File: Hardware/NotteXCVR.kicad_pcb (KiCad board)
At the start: 2 copper layers, 20.3 x 8.4 mm, 8 parts, among them J1 Bus_PCI_Express_x1, J2 GMI-10-2-1.27-G-10, U2 XC7A35T-CSG325

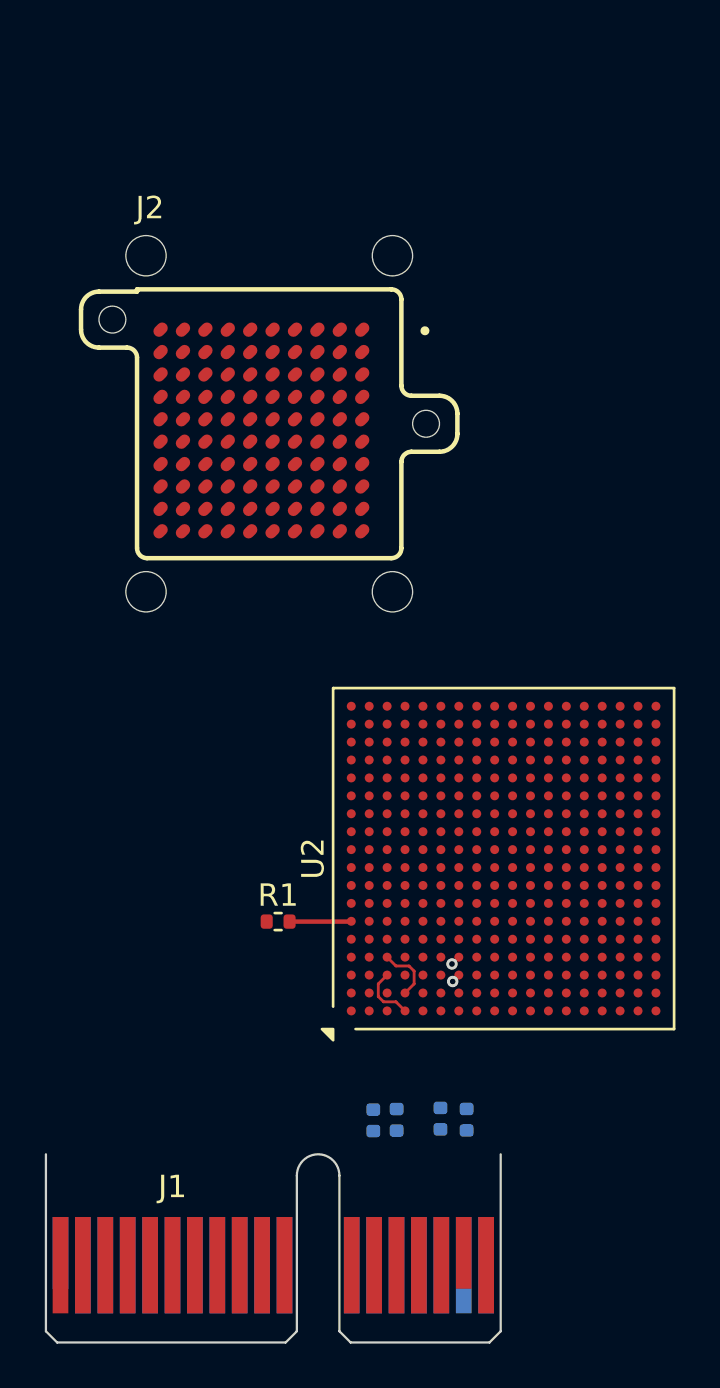
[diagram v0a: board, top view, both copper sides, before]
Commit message: Is this orientation better
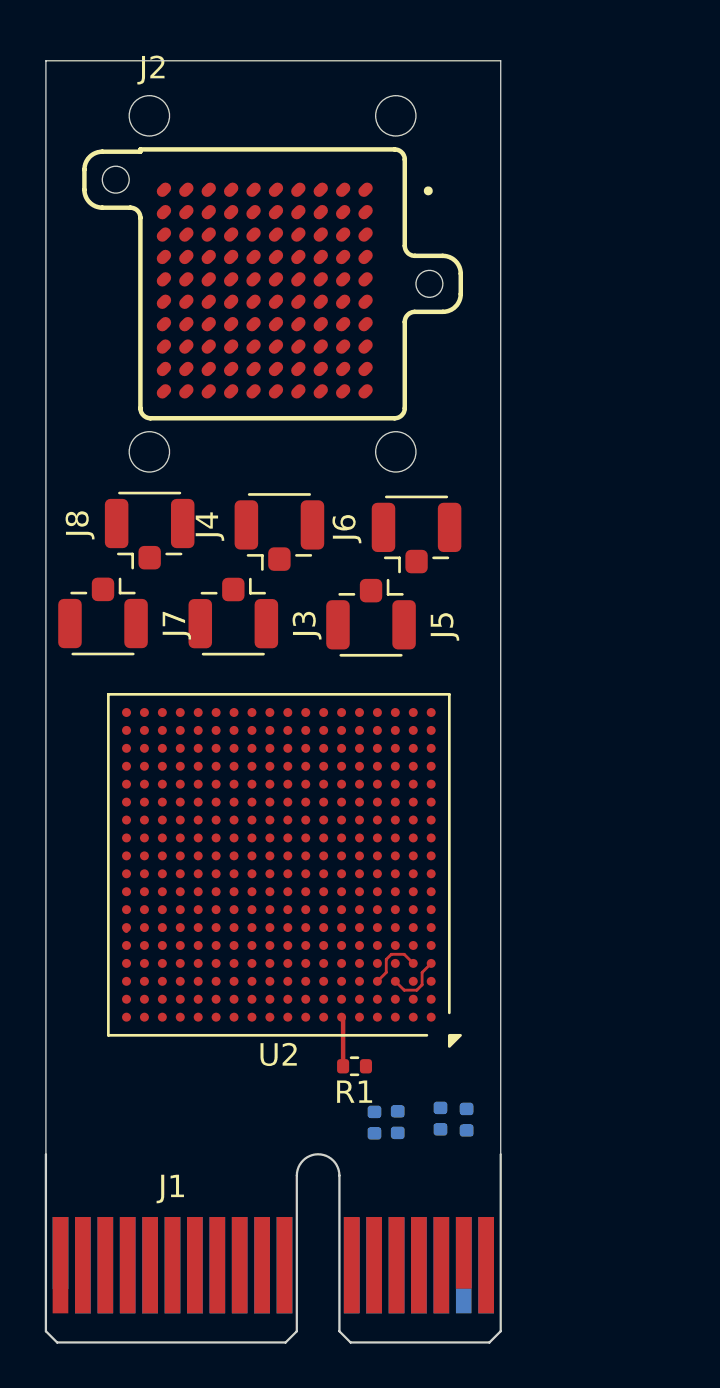
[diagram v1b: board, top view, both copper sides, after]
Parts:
- added J3: Conn_Coaxial, Connector_Coaxial:U.FL_Hirose_U.FL-R-SMT-1_Vertical, F.Cu at (85.1, 74.1)
- added J4: Conn_Coaxial, Connector_Coaxial:U.FL_Hirose_U.FL-R-SMT-1_Vertical, F.Cu at (87.1, 69.7)
- added J5: Conn_Coaxial, Connector_Coaxial:U.FL_Hirose_U.FL-R-SMT-1_Vertical, F.Cu at (91.2, 74.1)
- added J6: Conn_Coaxial, Connector_Coaxial:U.FL_Hirose_U.FL-R-SMT-1_Vertical, F.Cu at (93.2, 69.8)
- added J7: Conn_Coaxial, Connector_Coaxial:U.FL_Hirose_U.FL-R-SMT-1_Vertical, F.Cu at (79.2, 74.1)
- added J8: Conn_Coaxial, Connector_Coaxial:U.FL_Hirose_U.FL-R-SMT-1_Vertical, F.Cu at (81.3, 69.6)
- moved U2 10.0 mm to (87.1, 84.9), turned to 180 degrees
- moved R1 7.30 mm to (90.5, 93.9), turned to 180 degrees
- moved J2 6.25 mm to (86.8, 58.9)
- moved C2 0.11 mm to (92.4, 96.3)
- moved C1 0.11 mm to (91.4, 96.4)
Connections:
- C3 pad 2: PCIE_RX_P -> PCIE_TX_P
- C4 pad 2: PCIE_RX_N -> PCIE_TX_N
- J1 pad B14: PCIE_TX_P -> PCIE_RX_P
- J1 pad B15: PCIE_TX_N -> PCIE_RX_N
- U2 pad A1: unconnected-(U2F-GND-PadA1) -> GND
- U2 pad A11: unconnected-(U2F-GND-PadA11) -> GND
- U2 pad A16: unconnected-(U2A-VCCO_15-PadA16) -> Net-(U2A-VCCO_15-PadA16)
- U2 pad A18: unconnected-(U2F-GND-PadA18) -> GND
- U2 pad A3: /FPGA_MGT/MGT_SMA_RX_N -> /FPGA_MGT/MGT_UFL_RX_N
- U2 pad A4: /FPGA_MGT/MGT_SMA_RX_P -> /FPGA_MGT/MGT_UFL_RX_P
- U2 pad A5: unconnected-(U2F-GND-PadA5) -> GND
- U2 pad A7: unconnected-(U2F-GND-PadA7) -> GND
- U2 pad A8: unconnected-(U2F-GND-PadA8) -> GND
- U2 pad B13: unconnected-(U2A-VCCO_15-PadB13) -> Net-(U2A-VCCO_15-PadA16)
- U2 pad B18: unconnected-(U2F-GND-PadB18) -> GND
- U2 pad B3: unconnected-(U2F-GND-PadB3) -> GND
- U2 pad B7: unconnected-(U2F-GND-PadB7) -> GND
- U2 pad B8: unconnected-(U2F-GND-PadB8) -> GND
- U2 pad C10: unconnected-(U2A-VCCO_15-PadC10) -> Net-(U2A-VCCO_15-PadA16)
- U2 pad C15: unconnected-(U2F-GND-PadC15) -> GND
- U2 pad C2: unconnected-(U2F-GND-PadC2) -> GND
- U2 pad C6: unconnected-(U2F-GND-PadC6) -> GND
- U2 pad C7: unconnected-(U2F-GND-PadC7) -> GND
- U2 pad D12: unconnected-(U2F-GND-PadD12) -> GND
- U2 pad D17: unconnected-(U2A-VCCO_15-PadD17) -> Net-(U2A-VCCO_15-PadA16)
- U2 pad D3: unconnected-(U2F-GND-PadD3) -> GND
- U2 pad D4: unconnected-(U2F-GND-PadD4) -> GND
- U2 pad D5: /FPGA_MGT/SMA_CLK_N -> /FPGA_MGT/UFL_CLK_N
- U2 pad D6: /FPGA_MGT/SMA_CLK_P -> /FPGA_MGT/UFL_CLK_P
- U2 pad D7: unconnected-(U2F-GND-PadD7) -> GND
- U2 pad E11: unconnected-(U2F-VCCBATT_0-PadE11) -> +1V8
- U2 pad E14: unconnected-(U2A-VCCO_15-PadE14) -> Net-(U2A-VCCO_15-PadA16)
- U2 pad E2: unconnected-(U2F-GND-PadE2) -> GND
- U2 pad E6: unconnected-(U2F-GND-PadE6) -> GND
- U2 pad E7: unconnected-(U2F-GND-PadE7) -> GND
- U2 pad E9: unconnected-(U2F-GND-PadE9) -> GND
- U2 pad F1: /FPGA_MGT/MGT_SMA_TX_N -> /FPGA_MGT/MGT_UFL_TX_N
- U2 pad F10: unconnected-(U2F-GND-PadF10) -> GND
- U2 pad F11: unconnected-(U2F-VCCBRAM-PadF11) -> +1V0
- U2 pad F16: unconnected-(U2F-GND-PadF16) -> GND
- U2 pad F2: /FPGA_MGT/MGT_SMA_TX_P -> /FPGA_MGT/MGT_UFL_TX_P
- U2 pad F4: unconnected-(U2F-GND-PadF4) -> GND
- U2 pad F6: unconnected-(U2F-GND-PadF6) -> GND
- U2 pad F7: unconnected-(U2F-VCCINT-PadF7) -> +1V0
- U2 pad F9: unconnected-(U2F-VCCINT-PadF9) -> +1V0
- U2 pad G1: unconnected-(U2F-GND-PadG1) -> GND
- U2 pad G10: unconnected-(U2F-VCCBRAM-PadG10) -> +1V0
- U2 pad G11: unconnected-(U2F-GND-PadG11) -> GND
- U2 pad G12: unconnected-(U2F-VCCAUX-PadG12) -> +1V8
- U2 pad G13: unconnected-(U2F-GND-PadG13) -> GND
- U2 pad G18: unconnected-(U2A-VCCO_15-PadG18) -> Net-(U2A-VCCO_15-PadA16)
- U2 pad G5: unconnected-(U2F-GND-PadG5) -> GND
- U2 pad G6: unconnected-(U2F-GND-PadG6) -> GND
- U2 pad G7: unconnected-(U2F-GND-PadG7) -> GND
- U2 pad G8: unconnected-(U2F-VCCINT-PadG8) -> +1V0
- U2 pad G9: unconnected-(U2F-GND-PadG9) -> GND
- U2 pad H10: unconnected-(U2F-GND-PadH10) -> GND
- U2 pad H11: unconnected-(U2F-VCCBRAM-PadH11) -> +1V0
- U2 pad H12: unconnected-(U2F-GND-PadH12) -> GND
- U2 pad H13: unconnected-(U2F-VCCAUX-PadH13) -> +1V8
- U2 pad H15: unconnected-(U2A-VCCO_15-PadH15) -> Net-(U2A-VCCO_15-PadA16)
- U2 pad H3: unconnected-(U2F-GND-PadH3) -> GND
- U2 pad H4: unconnected-(U2F-GND-PadH4) -> GND
- U2 pad H5: unconnected-(U2F-GND-PadH5) -> GND
- U2 pad H6: unconnected-(U2F-GND-PadH6) -> GND
- U2 pad H7: unconnected-(U2F-VCCINT-PadH7) -> +1V0
- U2 pad H8: unconnected-(U2F-GND-PadH8) -> GND
- U2 pad H9: unconnected-(U2F-VCCINT-PadH9) -> +1V0
- U2 pad J1: unconnected-(U2F-GND-PadJ1) -> GND
- U2 pad J10: unconnected-(U2F-VCCADC_0-PadJ10) -> +1V8
- U2 pad J11: unconnected-(U2F-GND-PadJ11) -> GND
- U2 pad J12: unconnected-(U2F-VCCINT-PadJ12) -> +1V0
- U2 pad J13: unconnected-(U2F-GND-PadJ13) -> GND
- U2 pad J17: unconnected-(U2F-GND-PadJ17) -> GND
- U2 pad J2: unconnected-(U2F-GND-PadJ2) -> GND
- U2 pad J3: unconnected-(U2F-GND-PadJ3) -> GND
- U2 pad J7: unconnected-(U2F-GND-PadJ7) -> GND
- U2 pad J8: unconnected-(U2F-VCCINT-PadJ8) -> +1V0
- U2 pad J9: unconnected-(U2F-GNDADC_0-PadJ9) -> GND
- U2 pad K11: unconnected-(U2F-VCCINT-PadK11) -> +1V0
- U2 pad K12: unconnected-(U2F-GND-PadK12) -> GND
- U2 pad K13: unconnected-(U2F-VCCAUX-PadK13) -> +1V8
- U2 pad K14: unconnected-(U2F-GND-PadK14) -> GND
- U2 pad K4: unconnected-(U2F-GND-PadK4) -> GND
- U2 pad K7: unconnected-(U2F-VCCINT-PadK7) -> +1V0
- U2 pad K8: unconnected-(U2F-GND-PadK8) -> GND
- U2 pad L1: unconnected-(U2F-GND-PadL1) -> GND
- U2 pad L11: unconnected-(U2F-GND-PadL11) -> GND
- U2 pad L12: unconnected-(U2F-VCCINT-PadL12) -> +1V0
- U2 pad L13: unconnected-(U2F-GND-PadL13) -> GND
- U2 pad L16: unconnected-(U2A-VCCO_14-PadL16) -> Net-(U2A-VCCO_14-PadL16)
- U2 pad L6: unconnected-(U2B-VCCO_34-PadL6) -> Net-(U2B-VCCO_34-PadL6)
- U2 pad L7: unconnected-(U2F-GND-PadL7) -> GND
- U2 pad L8: unconnected-(U2F-VCCINT-PadL8) -> +1V0
- U2 pad M11: unconnected-(U2F-VCCINT-PadM11) -> +1V0
- U2 pad M12: unconnected-(U2F-GND-PadM12) -> GND
- U2 pad M13: unconnected-(U2F-VCCAUX-PadM13) -> +1V8
- U2 pad M18: unconnected-(U2F-GND-PadM18) -> GND
- U2 pad M3: unconnected-(U2B-VCCO_34-PadM3) -> Net-(U2B-VCCO_34-PadL6)
- U2 pad M7: unconnected-(U2F-VCCINT-PadM7) -> +1V0
- U2 pad M8: unconnected-(U2F-GND-PadM8) -> GND
- U2 pad N10: unconnected-(U2F-VCCINT-PadN10) -> +1V0
- U2 pad N11: unconnected-(U2F-GND-PadN11) -> GND
- U2 pad N12: unconnected-(U2F-VCCINT-PadN12) -> +1V0
- U2 pad N13: unconnected-(U2F-GND-PadN13) -> GND
- U2 pad N15: unconnected-(U2F-GND-PadN15) -> GND
- U2 pad N5: unconnected-(U2F-GND-PadN5) -> GND
- U2 pad N7: unconnected-(U2F-GND-PadN7) -> GND
- U2 pad N8: unconnected-(U2F-VCCINT-PadN8) -> +1V0
- U2 pad N9: unconnected-(U2F-GND-PadN9) -> GND
- U2 pad P11: unconnected-(U2F-VCCINT-PadP11) -> +1V0
- U2 pad P12: unconnected-(U2F-GND-PadP12) -> GND
- U2 pad P13: unconnected-(U2F-VCCAUX-PadP13) -> +1V8
- U2 pad P17: unconnected-(U2A-VCCO_14-PadP17) -> Net-(U2A-VCCO_14-PadL16)
- U2 pad P2: unconnected-(U2F-GND-PadP2) -> GND
- U2 pad P7: unconnected-(U2B-VCCO_34-PadP7) -> Net-(U2B-VCCO_34-PadL6)
- U2 pad P8: unconnected-(U2F-GND-PadP8) -> GND
- U2 pad P9: unconnected-(U2F-VCCINT-PadP9) -> +1V0
- U2 pad R14: unconnected-(U2A-VCCO_14-PadR14) -> Net-(U2A-VCCO_14-PadL16)
- U2 pad R4: unconnected-(U2B-VCCO_34-PadR4) -> Net-(U2B-VCCO_34-PadL6)
- U2 pad R9: unconnected-(U2F-GND-PadR9) -> GND
- U2 pad T1: unconnected-(U2B-VCCO_34-PadT1) -> Net-(U2B-VCCO_34-PadL6)
- U2 pad T11: unconnected-(U2A-VCCO_14-PadT11) -> Net-(U2A-VCCO_14-PadL16)
- U2 pad T16: unconnected-(U2F-GND-PadT16) -> GND
- U2 pad T6: unconnected-(U2F-GND-PadT6) -> GND
- U2 pad U13: unconnected-(U2F-GND-PadU13) -> GND
- U2 pad U18: unconnected-(U2A-VCCO_14-PadU18) -> Net-(U2A-VCCO_14-PadL16)
- U2 pad U3: unconnected-(U2F-GND-PadU3) -> GND
- U2 pad U8: unconnected-(U2A-VCCO_14-PadU8) -> Net-(U2A-VCCO_14-PadL16)
- U2 pad V1: unconnected-(U2F-GND-PadV1) -> GND
- U2 pad V10: unconnected-(U2F-GND-PadV10) -> GND
- U2 pad V15: unconnected-(U2A-VCCO_14-PadV15) -> Net-(U2A-VCCO_14-PadL16)
- U2 pad V18: unconnected-(U2F-GND-PadV18) -> GND
- U2 pad V5: unconnected-(U2B-VCCO_34-PadV5) -> Net-(U2B-VCCO_34-PadL6)
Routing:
- net Net-(U2D-MGTRREF_216): track 2.76 -> 2.22 mm
- net PCIE_RX_P: track 0.43 -> 0.00 mm, vias 1 -> 0
- net PCIE_RX_N: track 0.41 -> 0.00 mm, vias 1 -> 0
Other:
- board size 20.3 x 8.4 mm -> 20.3 x 48.8 mm
